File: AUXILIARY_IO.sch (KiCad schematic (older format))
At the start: 33 parts, among them J3 Conn_01x05_Male, Q4 SSM3K35AMFV, Q5 SSM3K35AMFV, Q6 SSM3K35AMFV, Q7 SSM3K35AMFV, Q8 SSM3K35AMFV, U6 NP_CM1293A-04SO, U7 NP_CM1293A-04SO

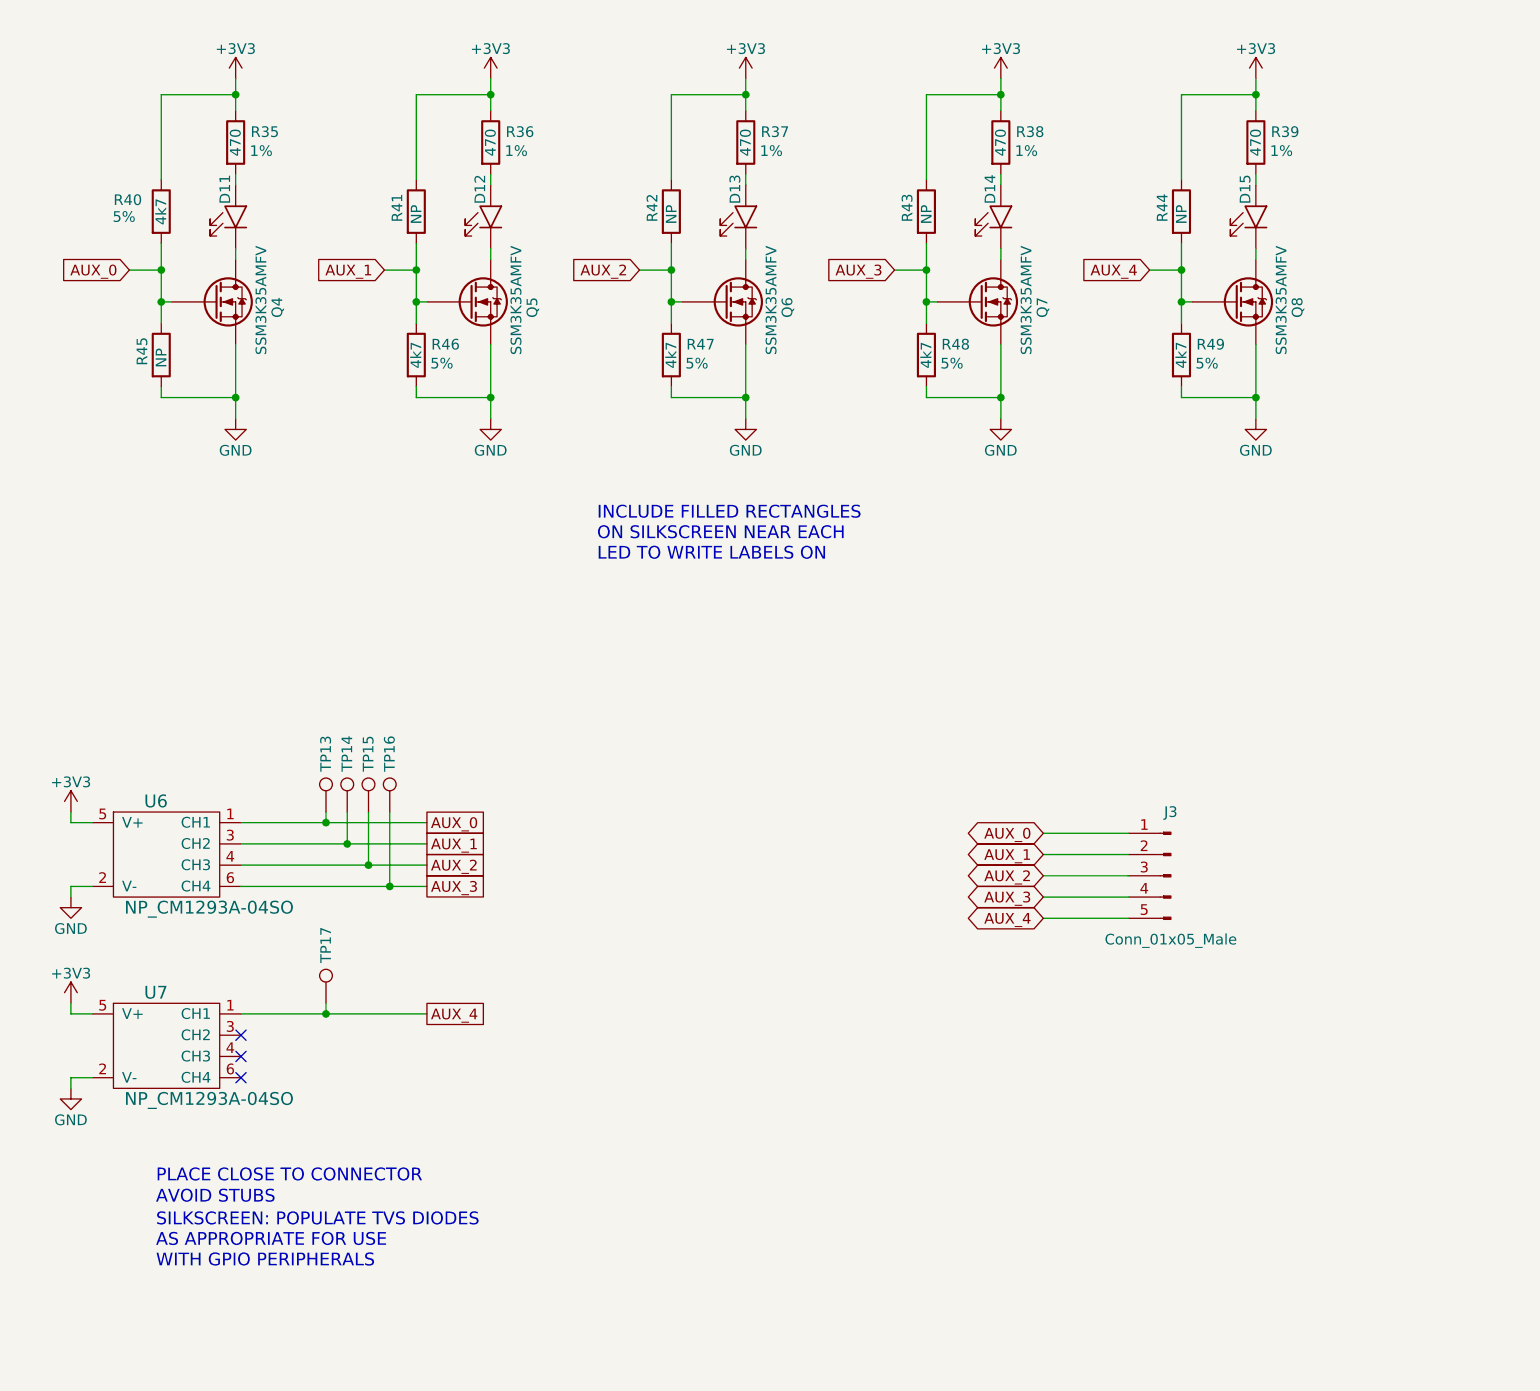
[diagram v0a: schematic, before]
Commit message: automated commit
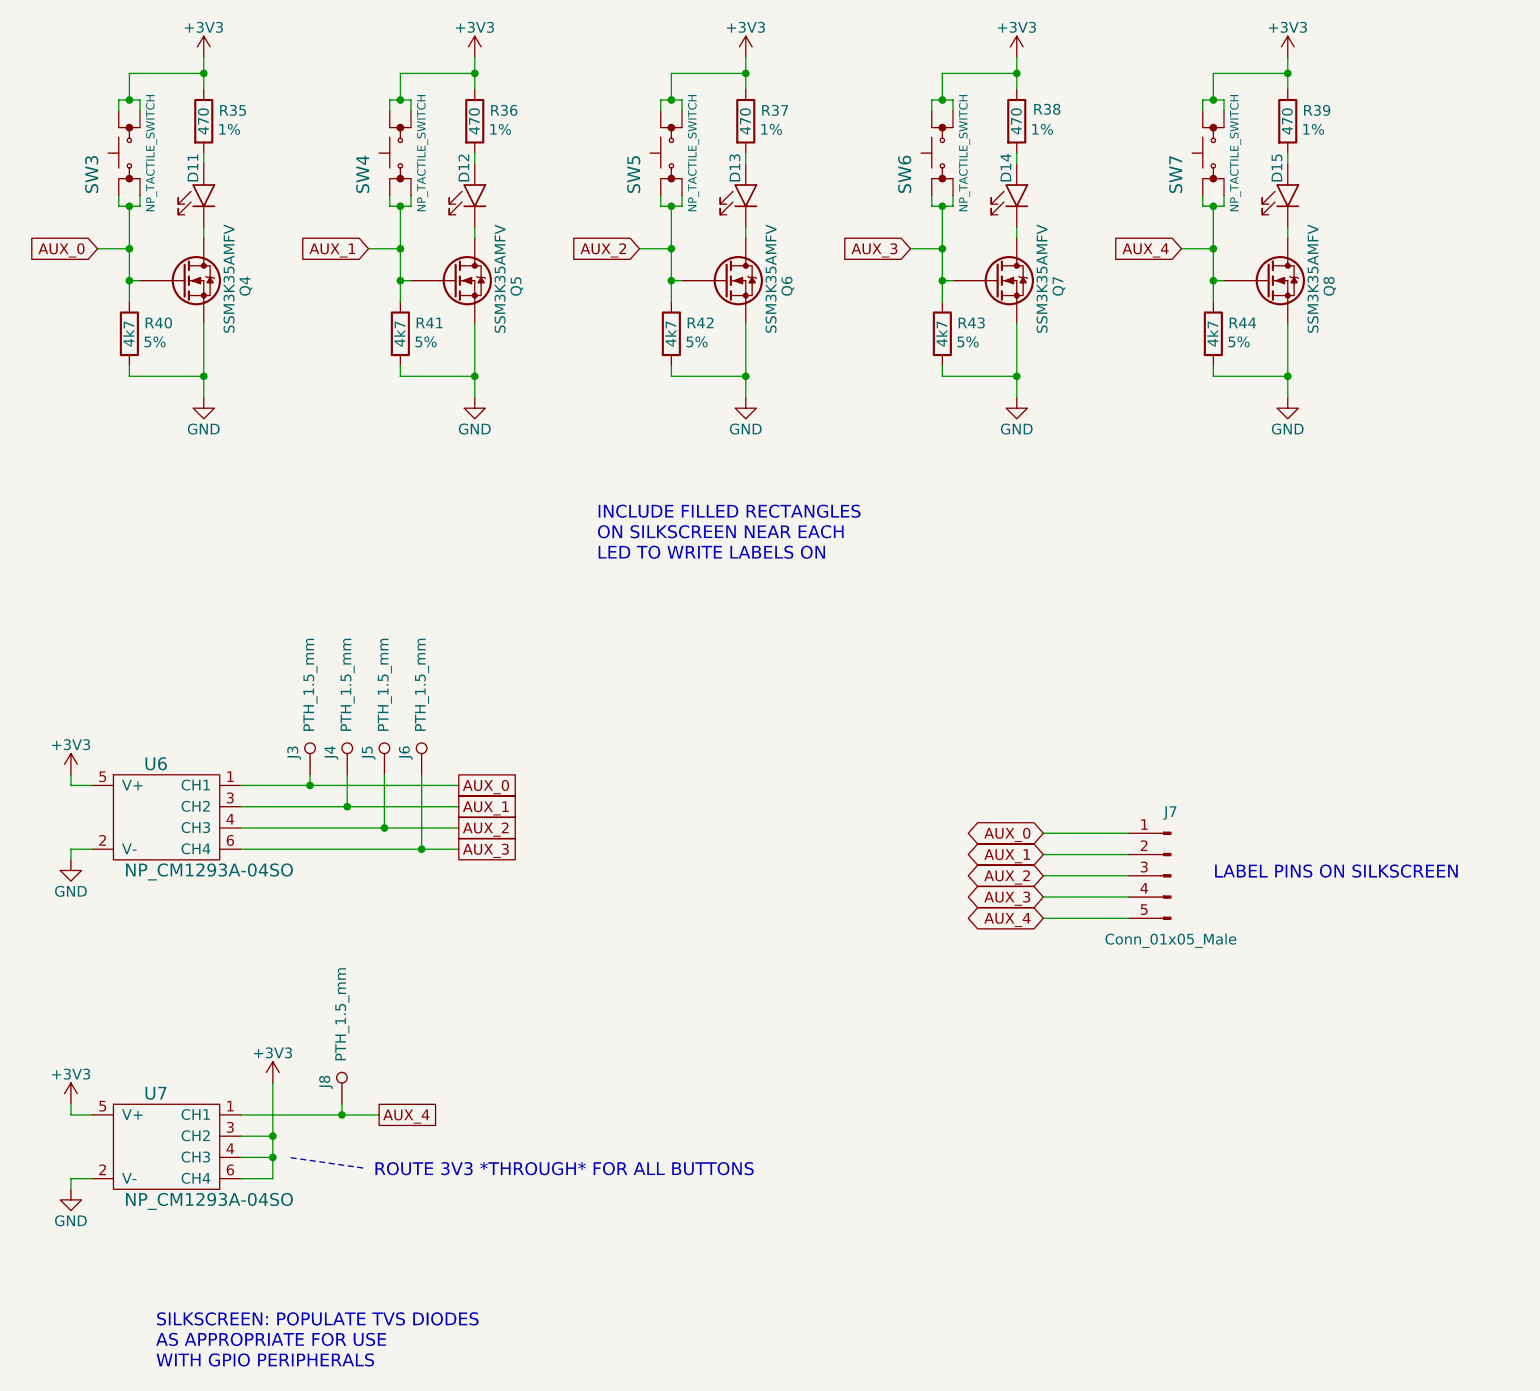
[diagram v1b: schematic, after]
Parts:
- removed D11: LED_GENERIC_0805, Diode_SMD:D_0805_2012Metric, symbol custom:LED_GENERIC_0805
- removed Q4: SSM3K35AMFV, symbol custom:SSM3K35AMFV
- removed R35: ‎RMCF0603FT470R‎, Resistor_SMD:R_0603_1608Metric, symbol custom:‎RMCF0603FT470R‎
- removed R40, R46, R47, R48: CRG0603F4K7, Resistor_SMD:R_0603_1608Metric, symbol custom:CRG0603F4K7
- removed R41, R42, R43, R44, R45: NP_R_0603, 0603, symbol custom:NP_R_0603
- removed TP13, TP14, TP15, TP16, TP17: TestPoint, symbol Connector:TestPoint
- added D15: LED_GENERIC_0805, Diode_SMD:D_0805_2012Metric, symbol custom:LED_GENERIC_0805
- added J3, J4, J5, J6, J8: PTH_1.5_mm, TestPoint:TestPoint_THTPad_D3.0mm_Drill1.5mm, symbol custom:PTH_1.5_mm
- added Q8: SSM3K35AMFV, symbol custom:SSM3K35AMFV
- added R39: ‎RMCF0603FT470R‎, Resistor_SMD:R_0603_1608Metric, symbol custom:‎RMCF0603FT470R‎
- added R41, R42, R43, R44: CRG0603F4K7, Resistor_SMD:R_0603_1608Metric, symbol custom:CRG0603F4K7
- added SW3, SW4, SW5, SW6, SW7: NP_TACTILE_SWITCH, CUSTOM:TACTILE_SWITCH, symbol custom:TACTILE_SWITCH
- renumbered D15 to D11, J3 to J7, Q8 to Q4, R39 to R35, R49 to R40
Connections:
- net +3V3: now also U7.3 (CH2), U7.4 (CH3), U7.6 (CH4), R39.1, SW3.2, SW4.2, SW5.2, SW6.2, SW7.2
- net AUX_0: now also Q4.1 (G), R40.1, J3.1, SW3.1
- net AUX_1: now also J4.1, R41.1, SW4.1
- net AUX_2: now also J5.1, R42.1, SW5.1
- net AUX_3: now also J6.1, R43.1, SW6.1
- net AUX_4: now also J8.1, Q8.1 (G), R44.1, SW7.1; no longer Q4.1 (G), R40.1
- net GND: now also Q8.2 (S), R41.2, R42.2, R43.2, R44.2
- new net: D15.2 (A), R39.2
- new net: D15.1 (K), Q8.3 (D)
- no-connect marks 3 -> 0
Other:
- note added: "LABEL PINS ON SILKSCREEN"
- note added: "ROUTE 3V3 *THROUGH* FOR ALL BUTTONS"
- note removed: "AVOID STUBS"
- note removed: "PLACE CLOSE TO CONNECTOR"
- moved on the sheet: D11, Q4, R35, R40, U6, U7

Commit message: automated commit
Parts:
- J7: footprint (none) -> Connector_PinHeader_2.54mm:PinHeader_1x05_P2.54mm_Vertical
- Q4, Q5, Q6, Q7, Q8: footprint (none) -> Package_TO_SOT_SMD:SOT-723
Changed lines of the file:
@@
 F 0 "J7" H 7500 5375 50  0000 C CNN
 F 1 "Conn_01x05_Male" H 7500 4775 50  0000 C CNN
-F 2 "" H 7500 5075 50  0001 C CNN
+F 2 "Connector_PinHeader_2.54mm:PinHeader_1x05_P2.54mm_Vertical" H 7500 5075 50  0001 C CNN
 F 3 "~" H 7500 5075 50  0001 C CNN
 	1    7500 5075
@@
 F 0 "Q4" V 3175 2200 50  0000 L BNN
 F 1 "SSM3K35AMFV" V 3100 2025 50  0000 L BNN
-F 2 "" H 3050 2150 50  0001 L BIN
+F 2 "Package_TO_SOT_SMD:SOT-723" H 3050 2150 50  0001 L BIN
 F 3 "datasheets/SSM3K35AMFV.pdf" H 3050 2125 50  0001 L BNN
 	1    2850 2275
@@
 F 0 "Q5" V 4450 2200 50  0000 L BNN
 F 1 "SSM3K35AMFV" V 4375 2025 50  0000 L BNN
-F 2 "" H 4325 2150 50  0001 L BIN
+F 2 "Package_TO_SOT_SMD:SOT-723" H 4325 2150 50  0001 L BIN
 F 3 "datasheets/SSM3K35AMFV.pdf" H 4325 2125 50  0001 L BNN
 	1    4125 2275
@@
 F 0 "Q6" V 5725 2200 50  0000 L BNN
 F 1 "SSM3K35AMFV" V 5650 2025 50  0000 L BNN
-F 2 "" H 5600 2150 50  0001 L BIN
+F 2 "Package_TO_SOT_SMD:SOT-723" H 5600 2150 50  0001 L BIN
 F 3 "datasheets/SSM3K35AMFV.pdf" H 5600 2125 50  0001 L BNN
 	1    5400 2275
@@
 F 0 "Q7" V 7000 2200 50  0000 L BNN
 F 1 "SSM3K35AMFV" V 6925 2025 50  0000 L BNN
-F 2 "" H 6875 2150 50  0001 L BIN
+F 2 "Package_TO_SOT_SMD:SOT-723" H 6875 2150 50  0001 L BIN
 F 3 "datasheets/SSM3K35AMFV.pdf" H 6875 2125 50  0001 L BNN
 	1    6675 2275
@@
 F 0 "Q8" V 8275 2200 50  0000 L BNN
 F 1 "SSM3K35AMFV" V 8200 2025 50  0000 L BNN
-F 2 "" H 8150 2150 50  0001 L BIN
+F 2 "Package_TO_SOT_SMD:SOT-723" H 8150 2150 50  0001 L BIN
 F 3 "datasheets/SSM3K35AMFV.pdf" H 8150 2125 50  0001 L BNN
 	1    7950 2275

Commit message: automated commit
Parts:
- U6, U7: footprint (none) -> custom:SOT-457; TEXT (none) -> CM1293A
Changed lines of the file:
@@
 F 0 "U6" H 2725 5050 60  0000 C CNN
 F 1 "NP_CM1293A-04SO" H 2975 4550 60  0000 C CNN
-F 2 "" H 2625 4700 60  0001 C CNN
-F 3 "datasheets/CM1293A-04SO-D.PDF" H 2775 4450 60  0001 C CNN
+F 2 "custom:SOT-457" H 2625 4700 60  0001 C CNN
+F 3 "~/datasheets/CM1293A-04SO-D.PDF" H 2775 4450 60  0001 C CNN
+F 4 "CM1293A" H 2775 4800 50  0001 C CNN "TEXT"
 	1    2775 4800
 	1    0    0    -1
@@
 F 0 "U7" H 2725 6600 60  0000 C CNN
 F 1 "NP_CM1293A-04SO" H 2975 6100 60  0000 C CNN
-F 2 "" H 2625 6250 60  0001 C CNN
-F 3 "datasheets/CM1293A-04SO-D.PDF" H 2775 6000 60  0001 C CNN
+F 2 "custom:SOT-457" H 2625 6250 60  0001 C CNN
+F 3 "~/datasheets/CM1293A-04SO-D.PDF" H 2775 6000 60  0001 C CNN
+F 4 "CM1293A" H 2775 6350 50  0001 C CNN "TEXT"
 	1    2775 6350
 	1    0    0    -1
